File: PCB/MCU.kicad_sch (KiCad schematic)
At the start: 2 parts, among them U5 STM32F405RGTx, Y1 24MHz

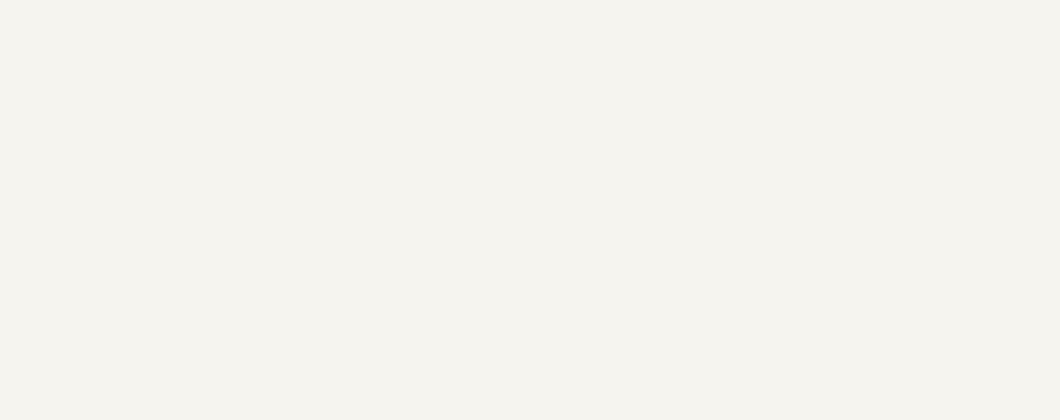
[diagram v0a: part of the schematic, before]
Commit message: PCB update - Minh
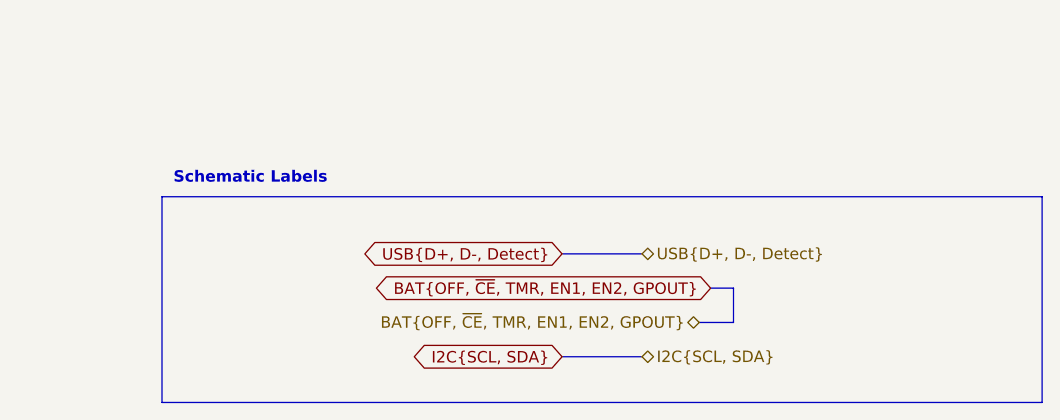
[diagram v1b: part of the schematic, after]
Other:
- note added: "Schematic Labels"
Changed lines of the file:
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@@
 (kicad_sch (version 20230121) (generator eeschema)
-  (paper "A4")
+  (paper "A3")
+  (bus (pts (xy 368.3 238.76) (xy 368.3 234.95))
+    (stroke (width 0) (type default))
+  )
+  (bus (pts (xy 368.3 234.95) (xy 365.76 234.95))
+    (stroke (width 0) (type default))
+  )
+  (bus (pts (xy 349.25 242.57) (xy 358.14 242.57))
+    (stroke (width 0) (type default))
+  )
+  (bus (pts (xy 349.25 231.14) (xy 358.14 231.14))
+    (stroke (width 0) (type default))
+  )
+  (bus (pts (xy 368.3 238.76) (xy 364.49 238.76))
+    (stroke (width 0) (type default))
+  )
+  (rectangle (start 304.8 224.79) (end 402.59 247.65)
+    (stroke (width 0) (type default))
+    (fill (type none))
+  )
+  (text "Schematic Labels" (at 306.07 223.52 0)
+    (effects (font (face "KiCad Font") (size 1.27 1.27) (thickness 0.254) bold) (justify left bottom))
+  )
+  (global_label "I2C{SCL, SDA}" (shape bidirectional) (at 349.25 242.57 180) (fields_autoplaced)
+    (effects (font (size 1.27 1.27)) (justify right))
+    (property "Intersheetrefs" "${INTERSHEET_REFS}" (at 331.7277 242.57 0)
+      (effects (font (size 1.27 1.27)) (justify right) hide)
+    )
+  )
+  (global_label "USB{D+, D-, Detect}" (shape bidirectional) (at 349.25 231.14 180) (fields_autoplaced)
+    (effects (font (size 1.27 1.27)) (justify right))
+    (property "Intersheetrefs" "${INTERSHEET_REFS}" (at 324.8333 231.14 0)
+      (effects (font (size 1.27 1.27)) (justify right) hide)
+    )
+  )
+  (global_label "BAT{OFF, ~{CE}, TMR, EN1, EN2, GPOUT}" (shape bidirectional) (at 365.76 234.95 180) (fields_autoplaced)
+    (effects (font (size 1.27 1.27)) (justify right))
+    (property "Intersheetrefs" "${INTERSHEET_REFS}" (at 325.6196 234.95 0)
+      (effects (font (size 1.27 1.27)) (justify right) hide)
+    )
+  )
+  (hierarchical_label "USB{D+, D-, Detect}" (shape bidirectional) (at 358.14 231.14 0) (fields_autoplaced)
+    (effects (font (size 1.27 1.27)) (justify left))
+  )
+  (hierarchical_label "I2C{SCL, SDA}" (shape bidirectional) (at 358.14 242.57 0) (fields_autoplaced)
+    (effects (font (size 1.27 1.27)) (justify left))
+  )
+  (hierarchical_label "BAT{OFF, ~{CE}, TMR, EN1, EN2, GPOUT}" (shape bidirectional) (at 364.49 238.76 180) (fields_autoplaced)
+    (effects (font (size 1.27 1.27)) (justify right))
+  )
   (symbol (lib_id "Device:Crystal") (at 173.99 54.61 0) (unit 1)
     (in_bom yes) (on_board yes) (dnp no) (fields_autoplaced)
@@
       (effects (font (size 1.27 1.27)) hide)
     )
+    (pin "1")
     (pin "2")
-    (pin "1")
     (instances
       (project "ECE477_PCBDesign"
@@
       (effects (font (size 1.27 1.27)) hide)
     )
-    (pin "44")
-    (pin "19")
-    (pin "35")
-    (pin "38")
-    (pin "41")
-    (pin "24")
+    (pin "1")
+    (pin "10")
+    (pin "11")
     (pin "12")
     (pin "13")
+    (pin "14")
+    (pin "15")
+    (pin "16")
+    (pin "17")
+    (pin "18")
+    (pin "19")
+    (pin "2")
+    (pin "20")
+    (pin "21")
+    (pin "22")
+    (pin "23")
+    (pin "24")
+    (pin "25")
+    (pin "26")
+    (pin "27")
+    (pin "28")
+    (pin "29")
+    (pin "3")
+    (pin "30")
+    (pin "31")
+    (pin "32")
+    (pin "33")
+    (pin "34")
+    (pin "35")
+    (pin "36")
+    (pin "37")
+    (pin "38")
+    (pin "39")
+    (pin "4")
+    (pin "40")
+    (pin "41")
+    (pin "42")
+    (pin "43")
+    (pin "44")
     (pin "45")
-    (pin "18")
-    (pin "25")
     (pin "46")
     (pin "47")
+    (pin "48")
+    (pin "49")
+    (pin "5")
+    (pin "50")
     (pin "51")
-    (pin "22")
-    (pin "14")
+    (pin "52")
     (pin "53")
     (pin "54")
+    (pin "55")
     (pin "56")
+    (pin "57")
     (pin "58")
-    (pin "48")
-    (pin "27")
     (pin "59")
-    (pin "33")
     (pin "6")
     (pin "60")
-    (pin "32")
-    (pin "40")
-    (pin "43")
-    (pin "10")
-    (pin "49")
-    (pin "57")
-    (pin "17")
-    (pin "23")
-    (pin "30")
-    (pin "50")
     (pin "61")
     (pin "62")
-    (pin "3")
-    (pin "11")
-    (pin "55")
     (pin "63")
-    (pin "4")
-    (pin "5")
     (pin "64")
-    (pin "28")
-    (pin "2")
-    (pin "37")
-    (pin "31")
-    (pin "34")
-    (pin "52")
-    (pin "21")
-    (pin "42")
-    (pin "20")
-    (pin "26")
-    (pin "16")
-    (pin "36")
-    (pin "29")
-    (pin "39")
-    (pin "15")
-    (pin "1")
     (pin "7")
+    (pin "8")
     (pin "9")
-    (pin "8")
     (instances
       (project "ECE477_PCBDesign"

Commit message: Revert "PCB update - Minh"
This reverts commit 0608947e49f54a64abc006b190e3b029bac40ad1.
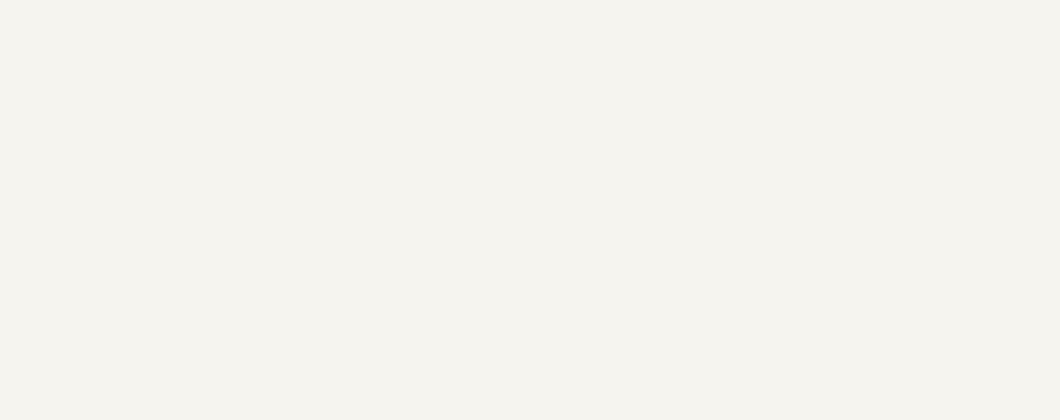
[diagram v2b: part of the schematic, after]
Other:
- note removed: "Schematic Labels"
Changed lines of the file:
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@@
 (kicad_sch (version 20230121) (generator eeschema)
-  (paper "A3")
-  (bus (pts (xy 368.3 238.76) (xy 368.3 234.95))
-    (stroke (width 0) (type default))
-  )
-  (bus (pts (xy 368.3 234.95) (xy 365.76 234.95))
-    (stroke (width 0) (type default))
-  )
-  (bus (pts (xy 349.25 242.57) (xy 358.14 242.57))
-    (stroke (width 0) (type default))
-  )
-  (bus (pts (xy 349.25 231.14) (xy 358.14 231.14))
-    (stroke (width 0) (type default))
-  )
-  (bus (pts (xy 368.3 238.76) (xy 364.49 238.76))
-    (stroke (width 0) (type default))
-  )
-  (rectangle (start 304.8 224.79) (end 402.59 247.65)
-    (stroke (width 0) (type default))
-    (fill (type none))
-  )
-  (text "Schematic Labels" (at 306.07 223.52 0)
-    (effects (font (face "KiCad Font") (size 1.27 1.27) (thickness 0.254) bold) (justify left bottom))
-  )
-  (global_label "I2C{SCL, SDA}" (shape bidirectional) (at 349.25 242.57 180) (fields_autoplaced)
-    (effects (font (size 1.27 1.27)) (justify right))
-    (property "Intersheetrefs" "${INTERSHEET_REFS}" (at 331.7277 242.57 0)
-      (effects (font (size 1.27 1.27)) (justify right) hide)
-    )
-  )
-  (global_label "USB{D+, D-, Detect}" (shape bidirectional) (at 349.25 231.14 180) (fields_autoplaced)
-    (effects (font (size 1.27 1.27)) (justify right))
-    (property "Intersheetrefs" "${INTERSHEET_REFS}" (at 324.8333 231.14 0)
-      (effects (font (size 1.27 1.27)) (justify right) hide)
-    )
-  )
-  (global_label "BAT{OFF, ~{CE}, TMR, EN1, EN2, GPOUT}" (shape bidirectional) (at 365.76 234.95 180) (fields_autoplaced)
-    (effects (font (size 1.27 1.27)) (justify right))
-    (property "Intersheetrefs" "${INTERSHEET_REFS}" (at 325.6196 234.95 0)
-      (effects (font (size 1.27 1.27)) (justify right) hide)
-    )
-  )
-  (hierarchical_label "USB{D+, D-, Detect}" (shape bidirectional) (at 358.14 231.14 0) (fields_autoplaced)
-    (effects (font (size 1.27 1.27)) (justify left))
-  )
-  (hierarchical_label "I2C{SCL, SDA}" (shape bidirectional) (at 358.14 242.57 0) (fields_autoplaced)
-    (effects (font (size 1.27 1.27)) (justify left))
-  )
-  (hierarchical_label "BAT{OFF, ~{CE}, TMR, EN1, EN2, GPOUT}" (shape bidirectional) (at 364.49 238.76 180) (fields_autoplaced)
-    (effects (font (size 1.27 1.27)) (justify right))
-  )
+  (paper "A4")
   (symbol (lib_id "Device:Crystal") (at 173.99 54.61 0) (unit 1)
     (in_bom yes) (on_board yes) (dnp no) (fields_autoplaced)
@@
       (effects (font (size 1.27 1.27)) hide)
     )
+    (pin "2")
     (pin "1")
-    (pin "2")
     (instances
       (project "ECE477_PCBDesign"
@@
       (effects (font (size 1.27 1.27)) hide)
     )
-    (pin "1")
-    (pin "10")
-    (pin "11")
+    (pin "44")
+    (pin "19")
+    (pin "35")
+    (pin "38")
+    (pin "41")
+    (pin "24")
     (pin "12")
     (pin "13")
-    (pin "14")
-    (pin "15")
-    (pin "16")
-    (pin "17")
+    (pin "45")
     (pin "18")
-    (pin "19")
-    (pin "2")
-    (pin "20")
-    (pin "21")
-    (pin "22")
-    (pin "23")
-    (pin "24")
     (pin "25")
-    (pin "26")
-    (pin "27")
-    (pin "28")
-    (pin "29")
-    (pin "3")
-    (pin "30")
-    (pin "31")
-    (pin "32")
-    (pin "33")
-    (pin "34")
-    (pin "35")
-    (pin "36")
-    (pin "37")
-    (pin "38")
-    (pin "39")
-    (pin "4")
-    (pin "40")
-    (pin "41")
-    (pin "42")
-    (pin "43")
-    (pin "44")
-    (pin "45")
     (pin "46")
     (pin "47")
-    (pin "48")
-    (pin "49")
-    (pin "5")
-    (pin "50")
     (pin "51")
-    (pin "52")
+    (pin "22")
+    (pin "14")
     (pin "53")
     (pin "54")
-    (pin "55")
     (pin "56")
-    (pin "57")
     (pin "58")
+    (pin "48")
+    (pin "27")
     (pin "59")
+    (pin "33")
     (pin "6")
     (pin "60")
+    (pin "32")
+    (pin "40")
+    (pin "43")
+    (pin "10")
+    (pin "49")
+    (pin "57")
+    (pin "17")
+    (pin "23")
+    (pin "30")
+    (pin "50")
     (pin "61")
     (pin "62")
+    (pin "3")
+    (pin "11")
+    (pin "55")
     (pin "63")
+    (pin "4")
+    (pin "5")
     (pin "64")
+    (pin "28")
+    (pin "2")
+    (pin "37")
+    (pin "31")
+    (pin "34")
+    (pin "52")
+    (pin "21")
+    (pin "42")
+    (pin "20")
+    (pin "26")
+    (pin "16")
+    (pin "36")
+    (pin "29")
+    (pin "39")
+    (pin "15")
+    (pin "1")
     (pin "7")
+    (pin "9")
     (pin "8")
-    (pin "9")
     (instances
       (project "ECE477_PCBDesign"
